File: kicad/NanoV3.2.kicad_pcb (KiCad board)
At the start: 2 copper layers, 43.2 x 17.8 mm, 23 parts, among them IC2 LM1117, IC3 ATMEGA328P-AU, P1 TTL, P2 OUT, P3 IN, Q1 BC237, Y1 16MHz

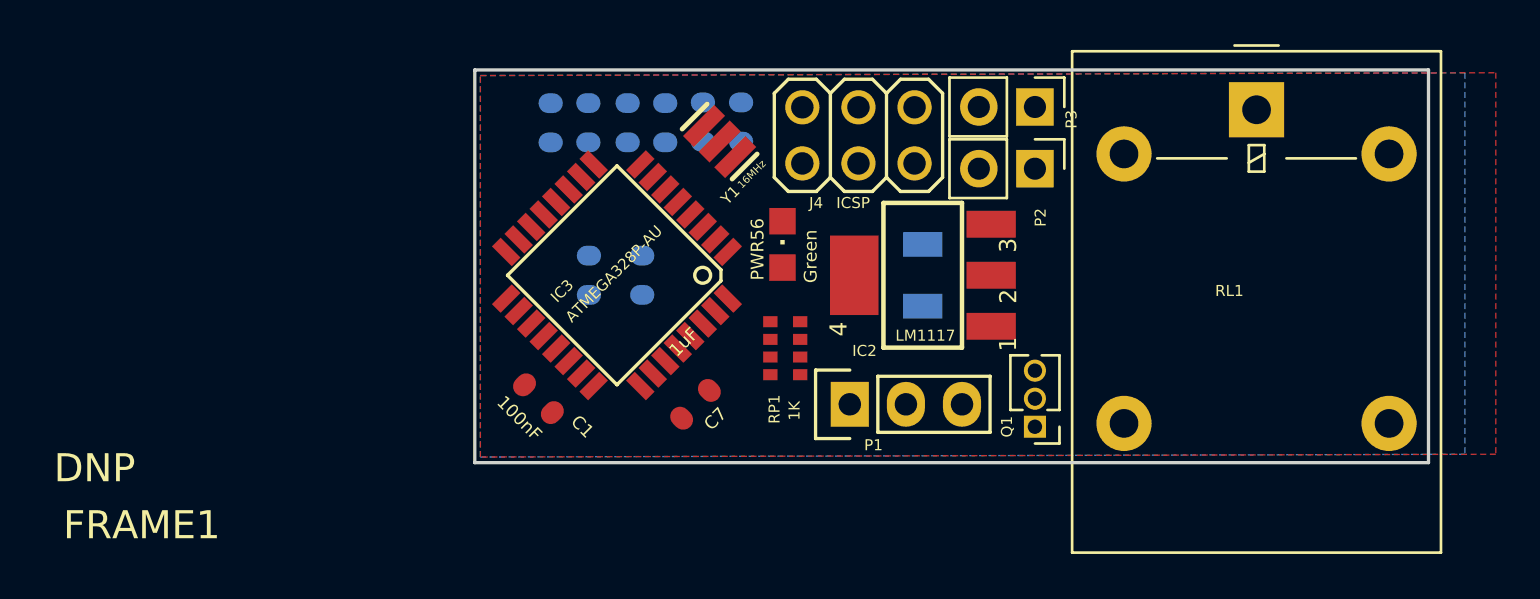
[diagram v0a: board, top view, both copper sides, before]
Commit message: finished layout
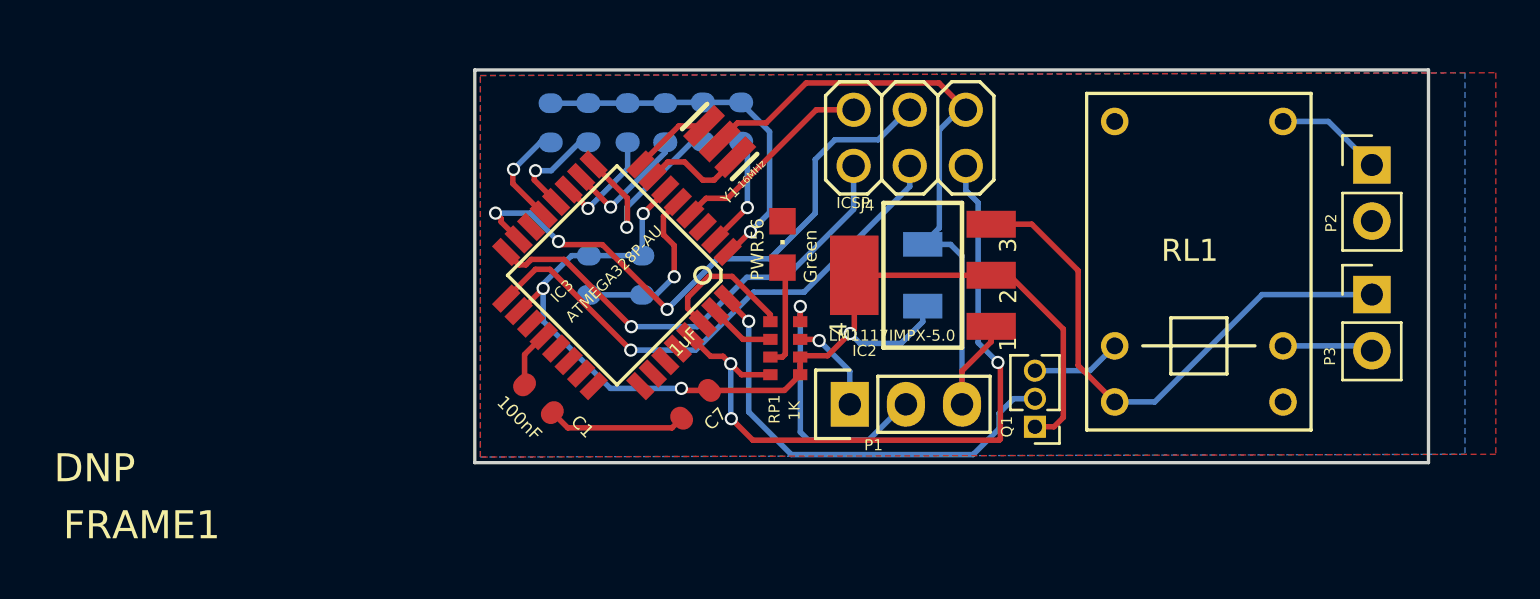
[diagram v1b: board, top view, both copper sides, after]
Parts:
- IC2: value LM1117 -> LM1117IMPX-5.0
- JP1, JP2, JP3, JP4, JP5, JP6: value Jumpper -> ~
- P3: value IN -> INPUT
- RL1: value FINDER-40.31 -> ~; footprint autoSwitch:Relay_SPDT_OMRON-G5LE-1 -> autoSwitch:Relay_HK4100F
- moved P3 17.5 mm to (167.5, 106.3), turned to 0 degrees
- moved P2 15.3 mm to (167.5, 100.4), turned to 0 degrees
- moved RL1 13.3 mm to (163.5, 111.1), turned to 90 degrees
- moved J4 2.32 mm to (146.6, 99.2)
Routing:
- net +5V: track 0.00 -> 61.0 mm, vias 0 -> 4
- net COM: track 0.00 -> 51.1 mm, vias 0 -> 1
- net /RESET: track 0.00 -> 32.5 mm, vias 0 -> 3
- net /D11/MOSI: track 0.00 -> 27.4 mm, vias 0 -> 3
- net VIN: track 0.00 -> 25.1 mm
- net /D13/SCK: track 0.00 -> 24.5 mm, vias 0 -> 1
- net /D12/MISO: track 0.00 -> 21.5 mm, vias 0 -> 1
- net /D2: track 0.00 -> 20.7 mm, vias 0 -> 1
- net /D3: track 0.00 -> 16.9 mm, vias 0 -> 1
- net Net-(P1-Pad2): track 0.00 -> 12.0 mm, vias 0 -> 1
- net /D5: track 0.00 -> 9.07 mm, vias 0 -> 1
- net /D0/RX: track 0.00 -> 6.64 mm
- net /D6: track 0.00 -> 5.87 mm, vias 0 -> 1
- net /D4: track 0.00 -> 5.23 mm, vias 0 -> 1
- net /D7: track 0.00 -> 4.97 mm, vias 0 -> 1
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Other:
- net class w0.5 added: clearance 0.4, trace_width 0.5, via_dia 1.2, via_drill 0.8
